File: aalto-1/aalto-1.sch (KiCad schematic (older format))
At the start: 6 parts

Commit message: Finished schematic rough draft
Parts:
- IC?: symbol RFPA5200:RFPA5200 -> aalto-1-rescue:RFPA5200-RFPA5200
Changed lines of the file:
@@
 $EndSheet
 $Comp
-L RFPA5200:RFPA5200 IC?
+L aalto-1-rescue:RFPA5200-RFPA5200 IC?
 U 1 1 6051A5FC
 P 2050 3350

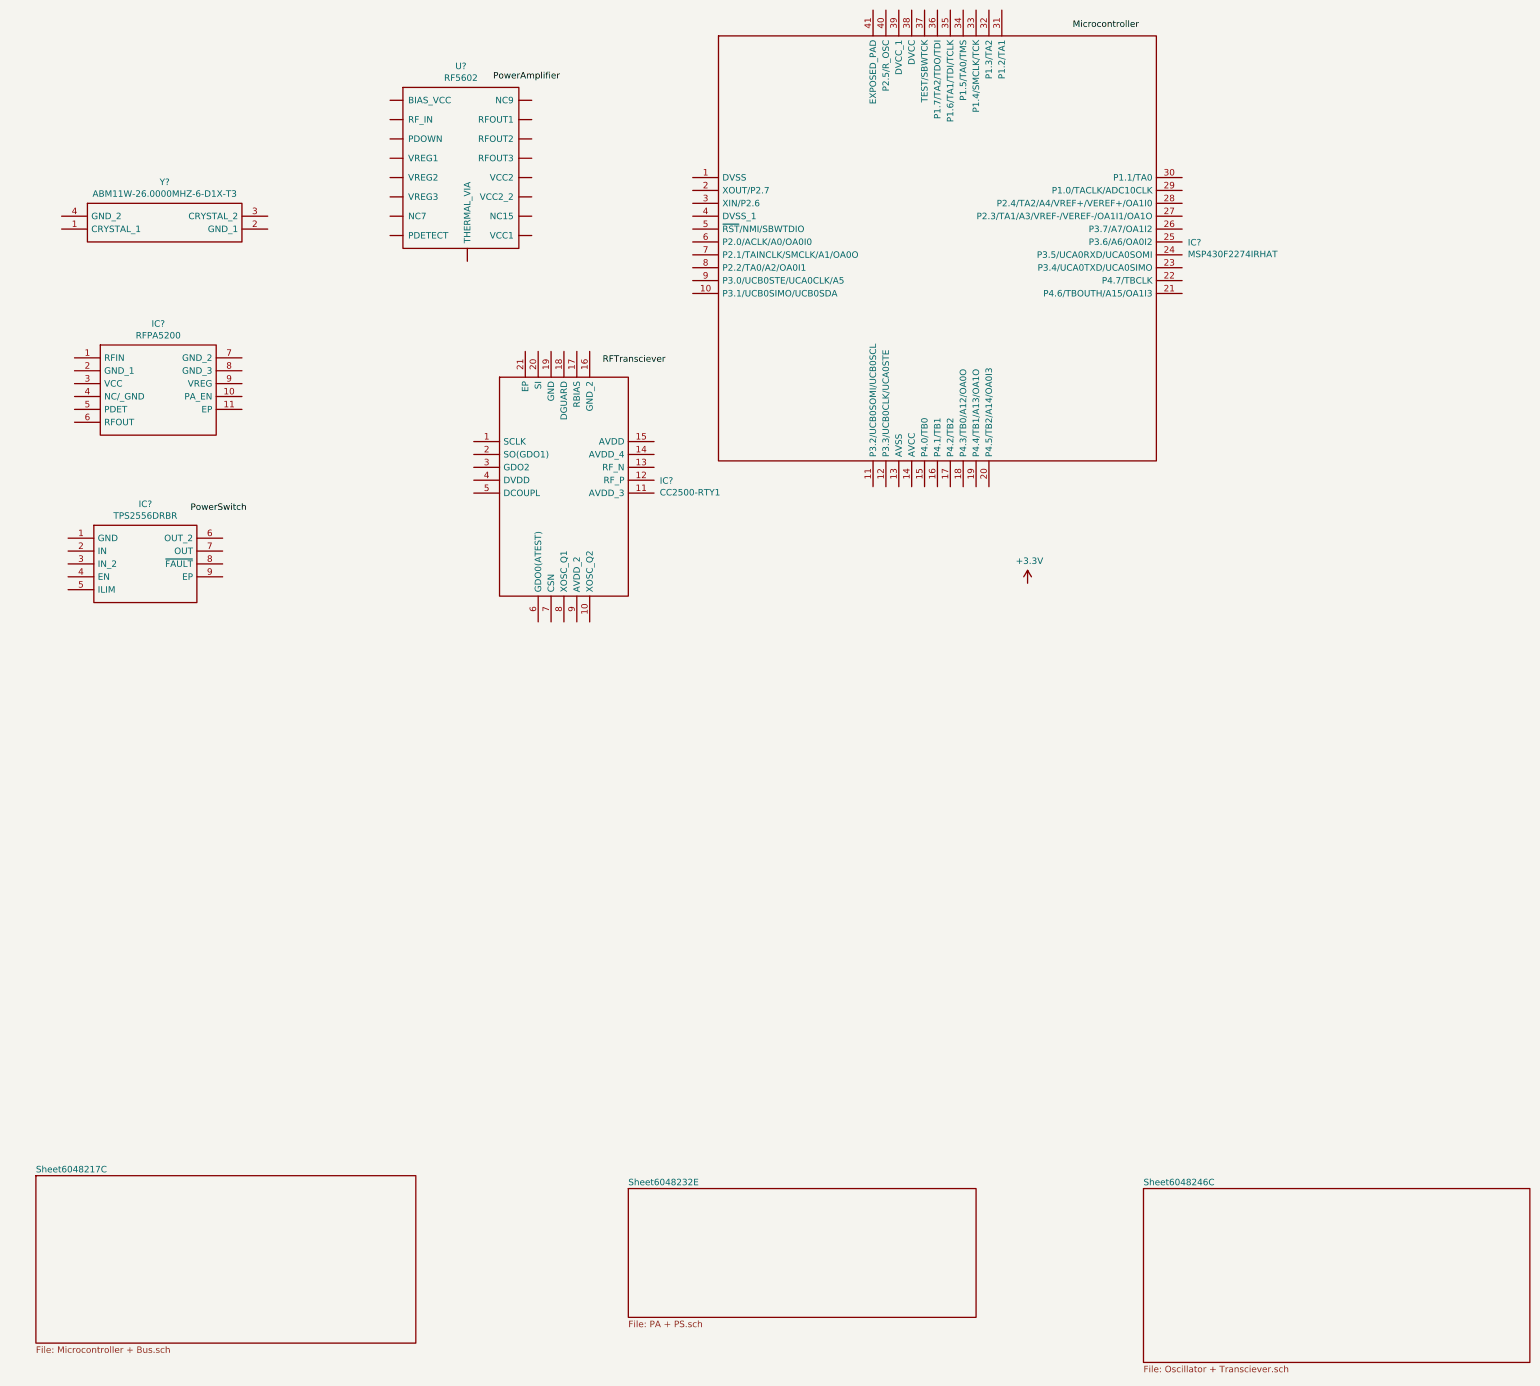
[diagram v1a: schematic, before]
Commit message: Labeling schematics
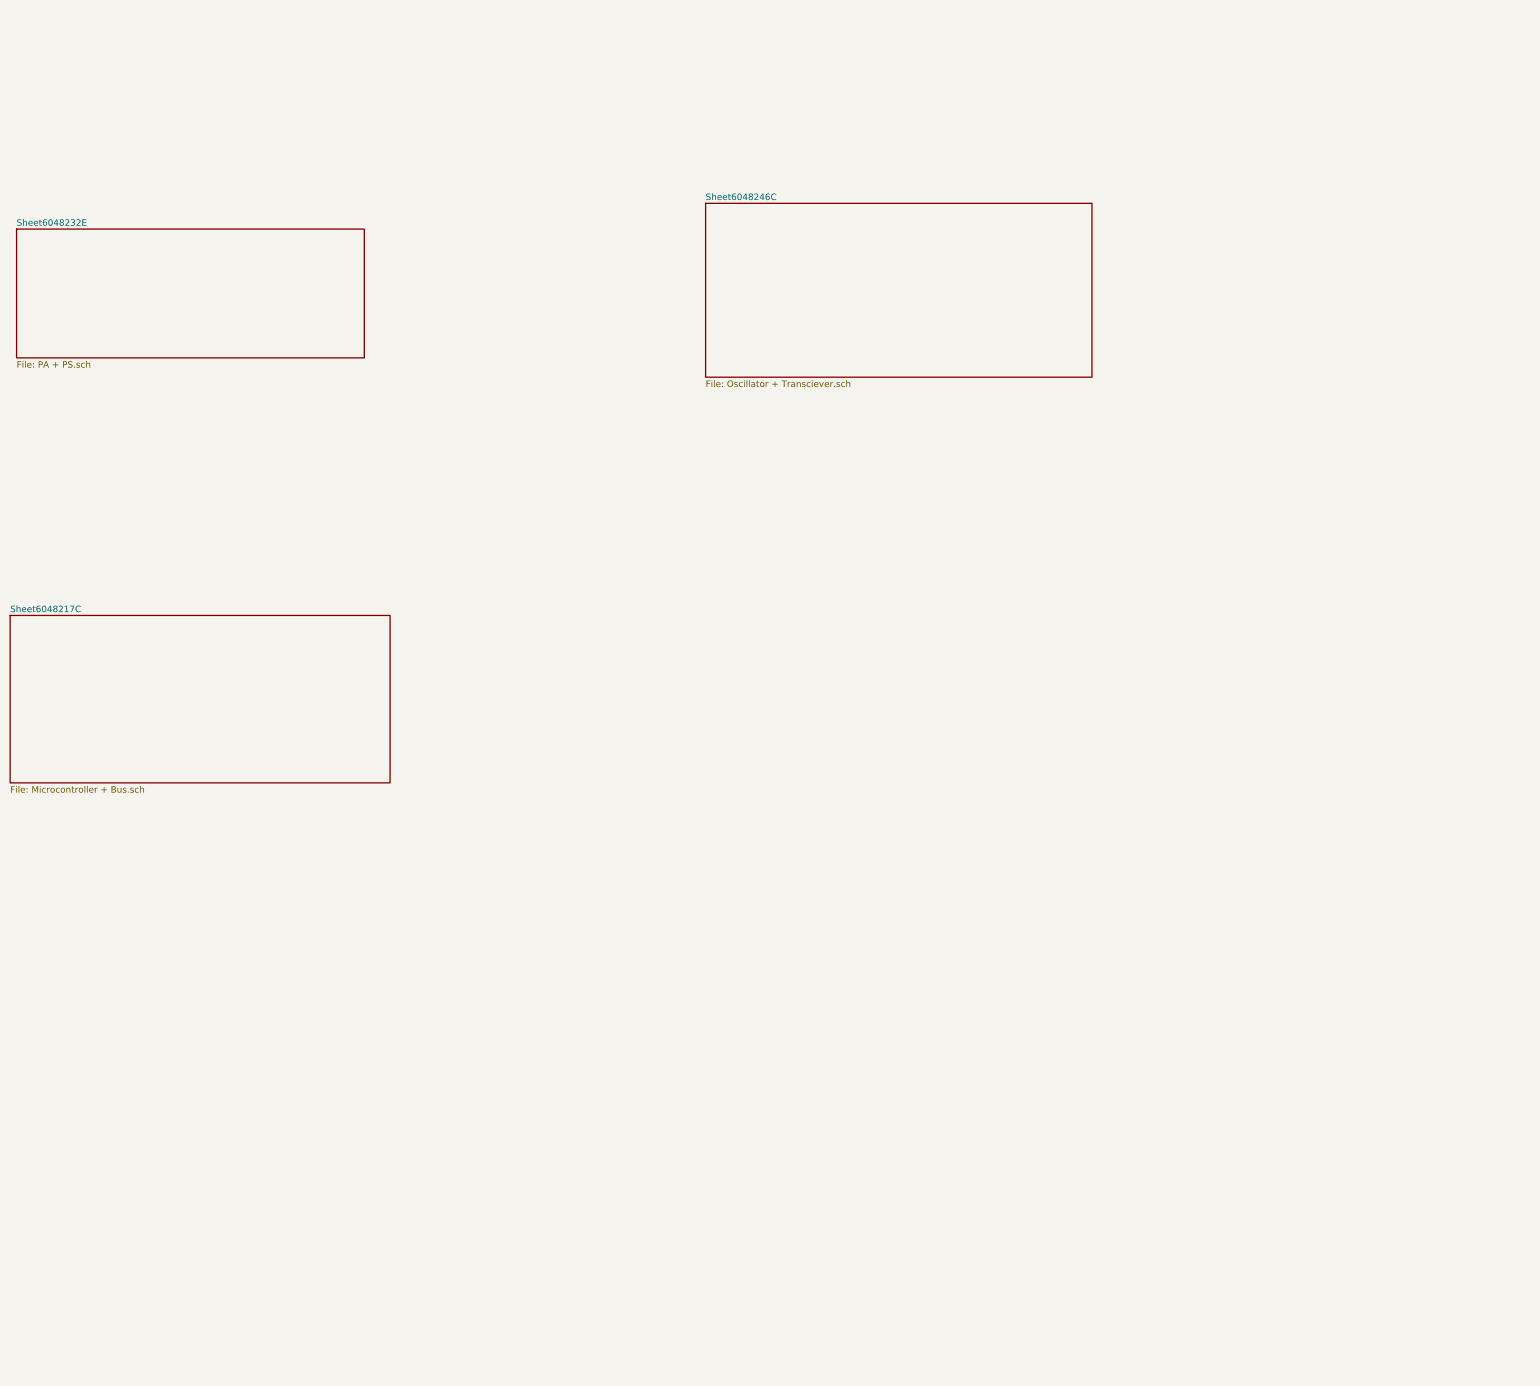
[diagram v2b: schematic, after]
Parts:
- removed IC?: CC2500-RTY1, QFN50P400X400X90-21N, symbol aalto-1-rescue:CC2500-RTY1-CC2500-RTY1
- removed IC?: MSP430F2274IRHAT, QFN50P600X600X100-41N-D, symbol aalto-1-rescue:MSP430F2274IRHAT-MSP430F2274IRHAT
- removed IC?: TPS2556DRBR, SON65P300X300X100-9N, symbol aalto-1-rescue:TPS2556DRBR-TPS2556DRBR
- removed IC?: RFPA5200, RFPA5200, symbol aalto-1-rescue:RFPA5200-RFPA5200
- removed U?: RF5602, symbol aalto-1-rescue:RF5602
- removed Y?: ABM11W-26.0000MHZ-6-D1X-T3, ABM11W300000MHZ4B1UT3, symbol aalto-1-rescue:ABM11W-26.0000MHZ-6-D1X-T3-ABM11W-26.0000MHZ-6-D1X-T3
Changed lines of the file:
@@
 Comment4 ""
 $EndDescr
-$Comp
-L aalto-1-rescue:+3.3V-power #PWR?
-U 1 1 600DD306
-P 9450 5100
-F 0 "#PWR?" H 9450 4950 50  0001 C CNN
-F 1 "+3.3V" H 9465 5273 50  0000 C CNN
-F 2 "" H 9450 5100 50  0001 C CNN
-F 3 "" H 9450 5100 50  0001 C CNN
-	1    9450 5100
-	1    0    0    -1
-$EndComp
-$Comp
-L aalto-1-rescue:CC2500-RTY1-CC2500-RTY1 IC?
-U 1 1 603BE95F
-P 5150 4000
-F 0 "IC?" H 6594 3696 50  0000 L CNN
-F 1 "CC2500-RTY1" H 6594 3605 50  0000 L CNN
-F 2 "QFN50P400X400X90-21N" H 6400 4500 50  0001 L CNN
-F 3 "" H 6400 4400 50  0001 L CNN
-F 4 "RF Transceiver" H 6400 4300 50  0001 L CNN "Description"
-F 5 "" H 6400 4200 50  0001 L CNN "Height"
-F 6 "Texas Instruments" H 6400 4100 50  0001 L CNN "Manufacturer_Name"
-F 7 "CC2500-RTY1" H 6400 4000 50  0001 L CNN "Manufacturer_Part_Number"
-F 8 "839-CC2500-RTY1" H 6400 3900 50  0001 L CNN "Mouser Part Number"
-F 9 "https://www.mouser.com/Search/Refine.aspx?Keyword=839-CC2500-RTY1" H 6400 3800 50  0001 L CNN "Mouser Price/Stock"
-F 10 "" H 6400 3700 50  0001 L CNN "Arrow Part Number"
-F 11 "" H 6400 3600 50  0001 L CNN "Arrow Price/Stock"
-	1    5150 4000
-	1    0    0    -1
-$EndComp
-$Comp
-L aalto-1-rescue:ABM11W-26.0000MHZ-6-D1X-T3-ABM11W-26.0000MHZ-6-D1X-T3 Y?
-U 1 1 603BF50A
-P 1950 2250
-F 0 "Y?" H 2750 2515 50  0000 C CNN
-F 1 "ABM11W-26.0000MHZ-6-D1X-T3" H 2750 2424 50  0000 C CNN
-F 2 "ABM11W300000MHZ4B1UT3" H 3400 2350 50  0001 L CNN
-F 3 "https://abracon.com/Resonators/ABM11W.pdf" H 3400 2250 50  0001 L CNN
-F 4 "Crystals 26MHz 6pF -40C +85C 10ppm" H 3400 2150 50  0001 L CNN "Description"
-F 5 "0" H 3400 2050 50  0001 L CNN "Height"
-F 6 "ABRACON" H 3400 1950 50  0001 L CNN "Manufacturer_Name"
-F 7 "ABM11W-26.0000MHZ-6-D1X-T3" H 3400 1850 50  0001 L CNN "Manufacturer_Part_Number"
-F 8 "815-11W26-6D1XT" H 3400 1750 50  0001 L CNN "Mouser Part Number"
-F 9 "https://www.mouser.co.uk/ProductDetail/ABRACON/ABM11W-260000MHZ-6-D1X-T3/?qs=5aG0NVq1C4z1GA6BiaLhDQ%3D%3D" H 3400 1650 50  0001 L CNN "Mouser Price/Stock"
-F 10 "" H 3400 1550 50  0001 L CNN "Arrow Part Number"
-F 11 "" H 3400 1450 50  0001 L CNN "Arrow Price/Stock"
-	1    1950 2250
-	1    0    0    -1
-$EndComp
-$Comp
-L aalto-1-rescue:TPS2556DRBR-TPS2556DRBR IC?
-U 1 1 603C13A8
-P 2000 4750
-F 0 "IC?" H 2600 5015 50  0000 C CNN
-F 1 "TPS2556DRBR" H 2600 4924 50  0000 C CNN
-F 2 "SON65P300X300X100-9N" H 3050 4850 50  0001 L CNN
-F 3 "http://www.ti.com/lit/gpn/TPS2556" H 3050 4750 50  0001 L CNN
-F 4 "Precision Adjustable Current-Limited Power-Distribution Switches  " H 3050 4650 50  0001 L CNN "Description"
-F 5 "" H 3050 4550 50  0001 L CNN "Height"
-F 6 "Texas Instruments" H 3050 4450 50  0001 L CNN "Manufacturer_Name"
-F 7 "TPS2556DRBR" H 3050 4350 50  0001 L CNN "Manufacturer_Part_Number"
-F 8 "595-TPS2556DRBR" H 3050 4250 50  0001 L CNN "Mouser Part Number"
-F 9 "https://www.mouser.co.uk/ProductDetail/Texas-Instruments/TPS2556DRBR?qs=PhbdE%2FyVlIdLuE1sx6iVjw%3D%3D" H 3050 4150 50  0001 L CNN "Mouser Price/Stock"
-F 10 "TPS2556DRBR" H 3050 4050 50  0001 L CNN "Arrow Part Number"
-F 11 "https://www.arrow.com/en/products/tps2556drbr/texas-instruments" H 3050 3950 50  0001 L CNN "Arrow Price/Stock"
-	1    2000 4750
-	1    0    0    -1
-$EndComp
-$Comp
-L aalto-1-rescue:MSP430F2274IRHAT-MSP430F2274IRHAT IC?
-U 1 1 603BFCBF
-P 6850 1950
-F 0 "IC?" H 10694 1446 50  0000 L CNN
-F 1 "MSP430F2274IRHAT" H 10694 1355 50  0000 L CNN
-F 2 "QFN50P600X600X100-41N-D" H 10500 3050 50  0001 L CNN
-F 3 "http://www.ti.com/lit/ds/symlink/msp430f2274.pdf" H 10500 2950 50  0001 L CNN
-F 4 "MSP430F2274IRHAT, 16 bit MSP430 Microcontroller 16MHz 32kb Flash, 1kb RAM, I2C LIN SPI 40-Pin VQFN" H 10500 2850 50  0001 L CNN "Description"
-F 5 "1" H 10500 2750 50  0001 L CNN "Height"
-F 6 "Texas Instruments" H 10500 2650 50  0001 L CNN "Manufacturer_Name"
-F 7 "MSP430F2274IRHAT" H 10500 2550 50  0001 L CNN "Manufacturer_Part_Number"
-F 8 "595-MSP430F2274IRHAT" H 10500 2450 50  0001 L CNN "Mouser Part Number"
-F 9 "https://www.mouser.com/Search/Refine.aspx?Keyword=595-MSP430F2274IRHAT" H 10500 2350 50  0001 L CNN "Mouser Price/Stock"
-F 10 "MSP430F2274IRHAT" H 10500 2250 50  0001 L CNN "Arrow Part Number"
-F 11 "https://www.arrow.com/en/products/msp430f2274irhat/texas-instruments" H 10500 2150 50  0001 L CNN "Arrow Price/Stock"
-	1    6850 1950
-	1    0    0    -1
-$EndComp
-$Comp
-L aalto-1-rescue:RF5602 U?
-U 1 1 603F2812
-P 5100 1900
-F 0 "U?" H 5050 2715 50  0000 C CNN
-F 1 "RF5602" H 5050 2624 50  0000 C CNN
-F 2 "" H 5350 1200 50  0001 C CNN
-F 3 "" H 5350 1200 50  0001 C CNN
-	1    5100 1900
-	1    0    0    -1
-$EndComp
-Text Label 5300 1200 0    50   ~ 0
-PowerAmplifier
-Text Label 9800 800  0    50   ~ 0
-Microcontroller
-Text Label 2950 4550 0    50   ~ 0
-PowerSwitch
-Text Label 6150 3400 0    50   ~ 0
-RFTransciever
 $Sheet
-S 1750 9700 2950 1300
+S 1550 5350 2950 1300
 U 6048217D
 F0 "Sheet6048217C" 50
@@
 $EndSheet
 $Sheet
-S 6350 9800 2700 1000
+S 1600 2350 2700 1000
 U 6048232F
 F0 "Sheet6048232E" 50
@@
 $EndSheet
 $Sheet
-S 10350 9800 3000 1350
+S 6950 2150 3000 1350
 U 6048246D
 F0 "Sheet6048246C" 50
 F1 "Oscillator + Transciever.sch" 50
 $EndSheet
-$Comp
-L aalto-1-rescue:RFPA5200-RFPA5200 IC?
-U 1 1 6051A5FC
-P 2050 3350
-F 0 "IC?" H 2700 3615 50  0000 C CNN
-F 1 "RFPA5200" H 2700 3524 50  0000 C CNN
-F 2 "RFPA5200" H 3200 3450 50  0001 L CNN
-F 3 "https://www.qorvo.com/products/d/da001012" H 3200 3350 50  0001 L CNN
-F 4 "RF Amplifier 2.4-2.5GHz Gain 33dB Pout 27dBm 5V" H 3200 3250 50  0001 L CNN "Description"
-F 5 "1.05" H 3200 3150 50  0001 L CNN "Height"
-F 6 "Qorvo" H 3200 3050 50  0001 L CNN "Manufacturer_Name"
-F 7 "RFPA5200" H 3200 2950 50  0001 L CNN "Manufacturer_Part_Number"
-F 8 "N/A" H 3200 2850 50  0001 L CNN "Mouser Part Number"
-F 9 "https://www.mouser.com/Search/Refine.aspx?Keyword=N%2FA" H 3200 2750 50  0001 L CNN "Mouser Price/Stock"
-F 10 "" H 3200 2650 50  0001 L CNN "Arrow Part Number"
-F 11 "" H 3200 2550 50  0001 L CNN "Arrow Price/Stock"
-	1    2050 3350
-	1    0    0    -1
-$EndComp
 $EndSCHEMATC
